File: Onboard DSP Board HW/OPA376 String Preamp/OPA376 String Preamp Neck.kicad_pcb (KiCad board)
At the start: 2 copper layers, 28.4 x 89.9 mm, 49 parts, among them J1 Input, J10 Input, J14 Input, J5 Input, U1 OPA376xxDCK, U2 OPA376xxDCK, U3 OPA376xxDCK, U4 OPA376xxDCK

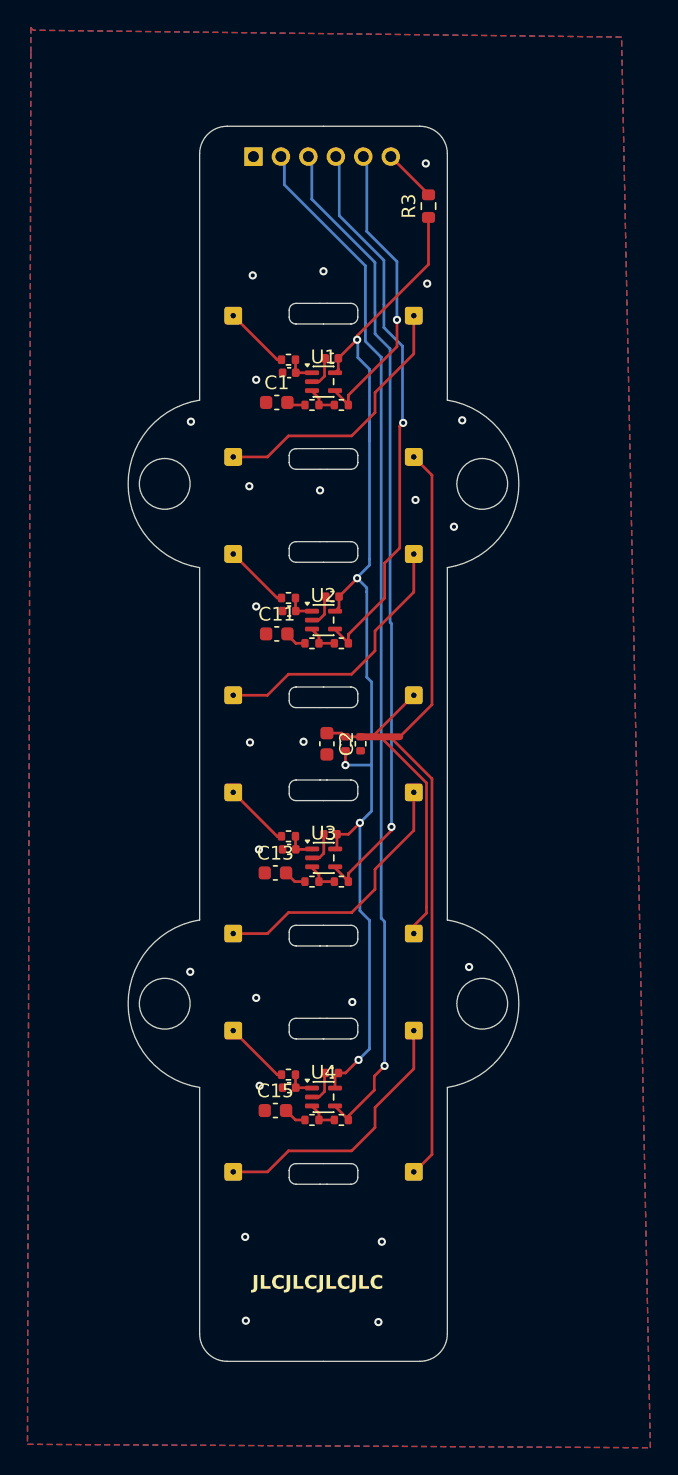
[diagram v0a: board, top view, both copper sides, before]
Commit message: WIP
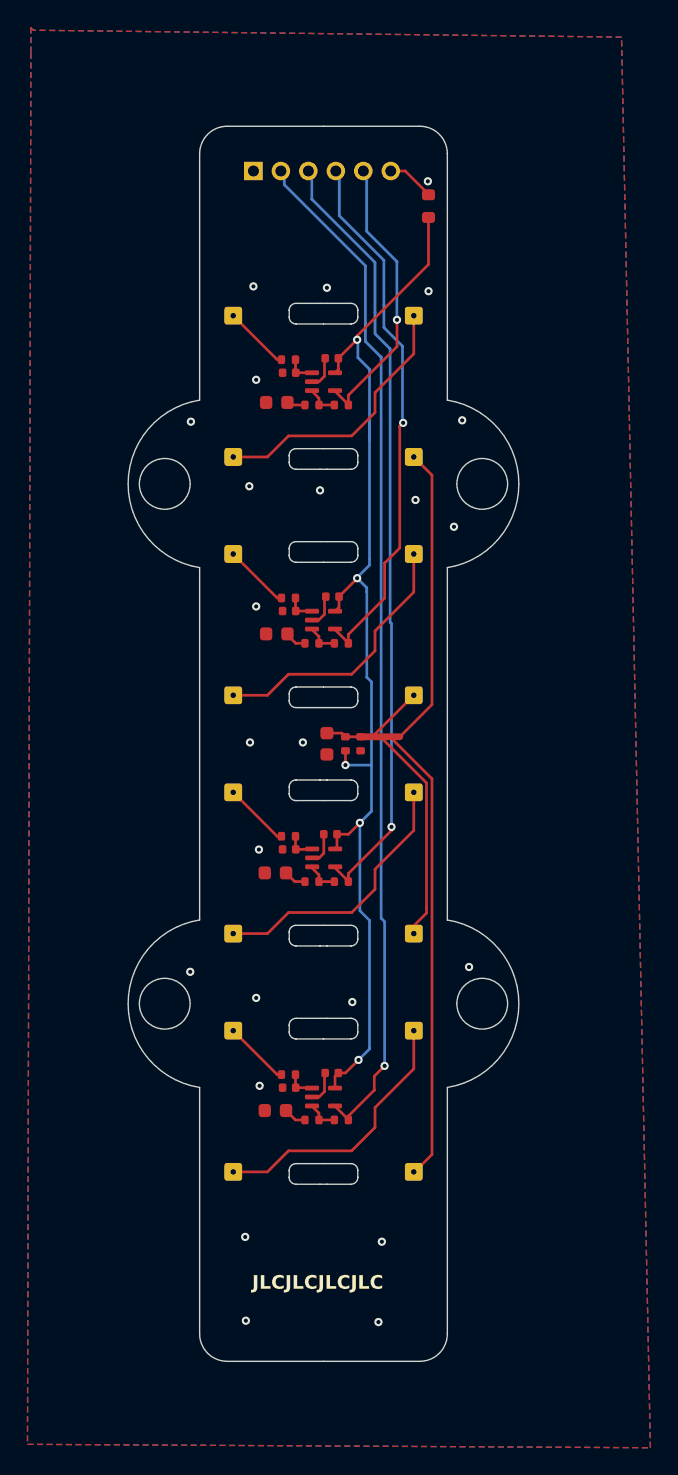
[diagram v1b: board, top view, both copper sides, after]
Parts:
- U1, U2, U3, U4: value OPA376xxDCK -> OPA376AIDCKT
- moved J9 1.05 mm to (94.9, 58.3)
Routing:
- net /SIngle FET preamp3/Output: track 75.8 -> 74.7 mm
- net /SIngle FET preamp1/Output: track 40.5 -> 39.5 mm
- net /SIngle FET preamp/Output: track 22.0 -> 20.9 mm
- net /SIngle FET preamp2/Output: track 58.0 -> 56.9 mm
- net GND: vias 22 -> 24
- net (no net): vias 2 -> 0
